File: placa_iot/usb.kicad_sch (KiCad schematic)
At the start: 9 parts, among them J5 USB4105-GF-A-120

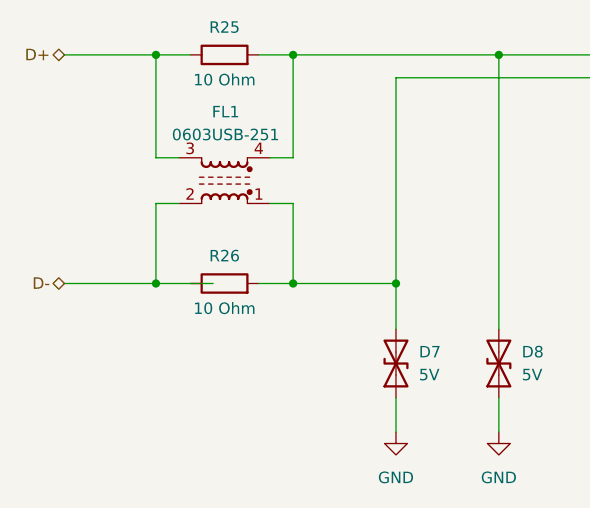
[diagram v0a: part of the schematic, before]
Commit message: Esquemático acabado
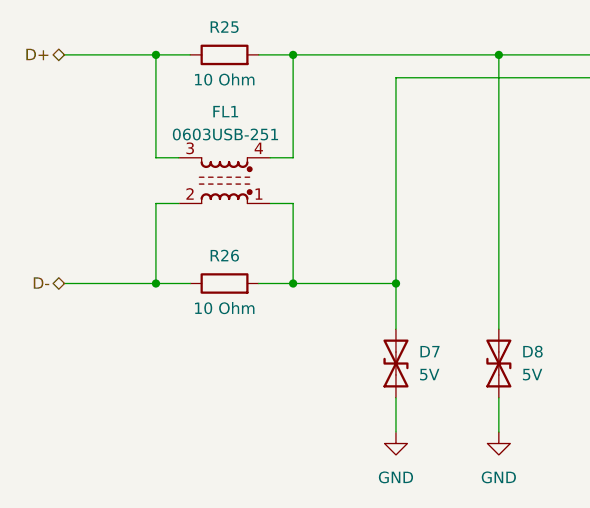
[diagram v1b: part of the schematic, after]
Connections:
- net D-: now also R26.1
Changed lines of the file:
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@@
+	)
+	(junction
+		(at 140.97 120.65)
+		(diameter 0)
+		(color 0 0 0 0)
+	)
+	(junction
+		(at 162.56 63.5)
+		(diameter 0)
+		(color 0 0 0 0)
+	)
+	(junction
+		(at 106.68 81.28)
+		(diameter 0)
+		(color 0 0 0 0)
+	)
+	(junction
+		(at 83.82 106.68)
+		(diameter 0)
+		(color 0 0 0 0)
+	)
+	(junction
+		(at 168.91 63.5)
+		(diameter 0)
+		(color 0 0 0 0)
+	)
+	(junction
+		(at 83.82 81.28)
+		(diameter 0)
+		(color 0 0 0 0)
+	)
+	(junction
+		(at 68.58 81.28)
+		(diameter 0)
+		(color 0 0 0 0)
 	)
 	(junction
 		(at 68.58 106.68)
-		(diameter 0)
-		(color 0 0 0 0)
-	)
-	(junction
-		(at 140.97 120.65)
-		(diameter 0)
-		(color 0 0 0 0)
-	)
-	(junction
-		(at 162.56 63.5)
-		(diameter 0)
-		(color 0 0 0 0)
-	)
-	(junction
-		(at 106.68 81.28)
-		(diameter 0)
-		(color 0 0 0 0)
-	)
-	(junction
-		(at 83.82 106.68)
-		(diameter 0)
-		(color 0 0 0 0)
-	)
-	(junction
-		(at 168.91 63.5)
-		(diameter 0)
-		(color 0 0 0 0)
-	)
-	(junction
-		(at 83.82 81.28)
-		(diameter 0)
-		(color 0 0 0 0)
-	)
-	(junction
-		(at 68.58 81.28)
 		(diameter 0)
 		(color 0 0 0 0)
@@
 	(wire
 		(pts
-			(xy 68.58 106.68) (xy 74.93 106.68)
-		)
-		(stroke
-			(width 0)
-			(type default)
-		)
-	)
-	(wire
-		(pts
 			(xy 68.58 81.28) (xy 72.39 81.28)
 		)
@@
 		)
 		(stroke
+			(width 0)
+			(type default)
+		)
+	)
+	(wire
+		(pts
+			(xy 68.58 106.68) (xy 72.39 106.68)
+		)
+		(stroke

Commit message: Layout iniciado y resolución de errores de huellas
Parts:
- J5: footprint connectors:CONN_SMT_RH_USBC_P0.50MM_P16 -> Connectors:CONN_SMT_RH_USBC_P0.50MM_P16
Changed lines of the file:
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@@
 			)
 		)
-		(property "Footprint" "connectors:CONN_SMT_RH_USBC_P0.50MM_P16"
+		(property "Footprint" "Connectors:CONN_SMT_RH_USBC_P0.50MM_P16"
 			(at 193.04 67.31 0)
 			(hide yes)
